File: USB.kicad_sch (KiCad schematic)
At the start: 40 parts, among them J5 USB_C_Receptacle, J6 USB_C_Receptacle, Q1 DMN32D2LFB4, Q2 DMN32D2LFB4, U10 TPD4EUSB30, U11 TPD4EUSB30, U12 TPD4EUSB30, U14 TPD4EUSB30, U15 TS3USB221, U17 TS3USB221, U19 TS3USB221, U20 TPD6S300A, U21 TPD6S300A, U7 FUSB340TMX, U9 FUSB340TMX

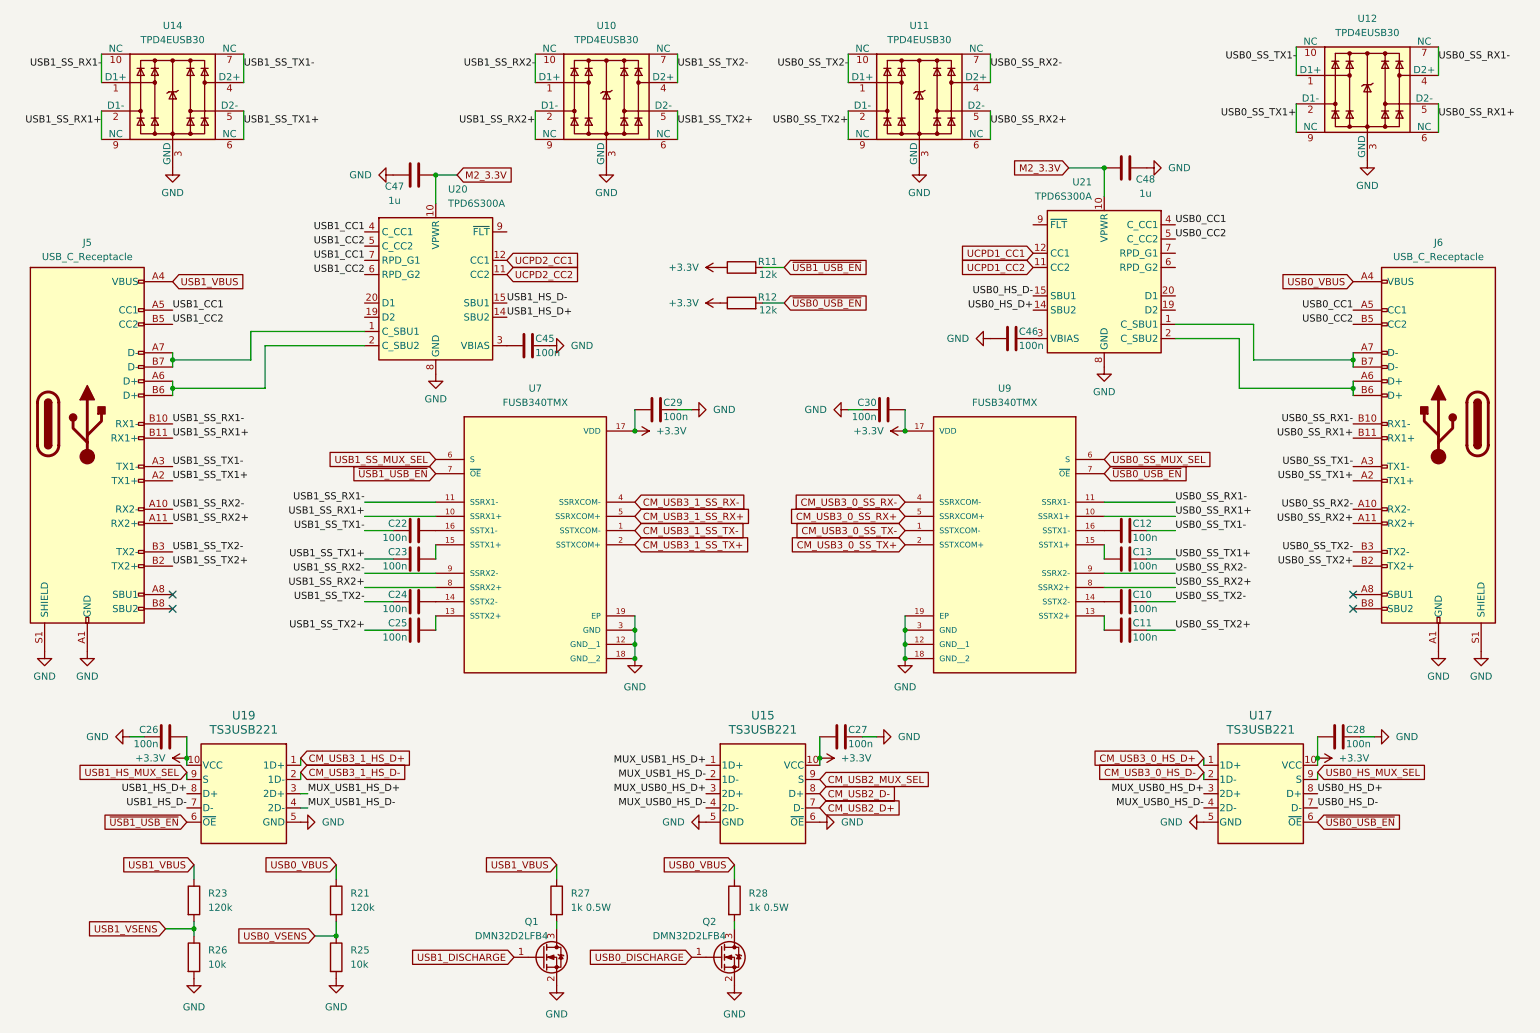
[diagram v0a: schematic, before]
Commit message: WIP
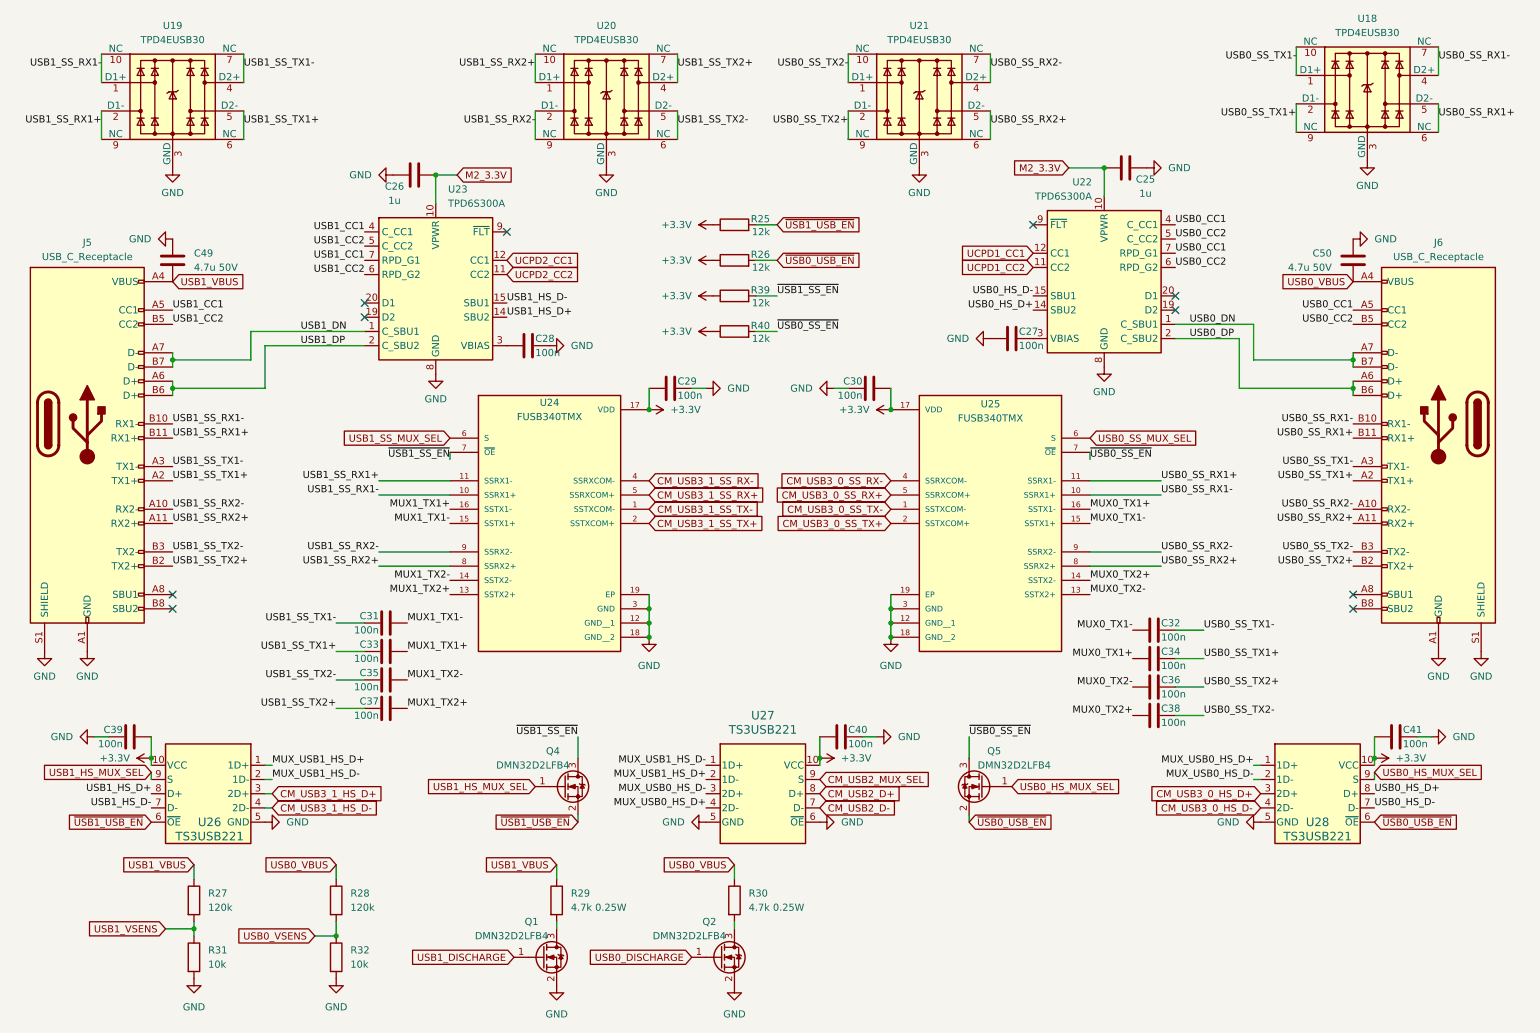
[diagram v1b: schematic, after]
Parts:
- removed C10, C11, C12, C13, C22, C23, C24, C25: 100n, Capacitor_SMD:C_0402_1005Metric, symbol Device:C
- added C31, C32, C33, C34, C35, C36, C37, C38: 100n, Capacitor_SMD:C_0402_1005Metric, symbol Device:C
- added C49, C50: 4.7u 50V, Capacitor_SMD:C_0805_2012Metric, symbol Device:C
- added Q4, Q5: DMN32D2LFB4, Package_DFN_QFN:Diodes_DFN1006-3, symbol Device:Q_NMOS_GSD
- added R39, R40: 12k, Resistor_SMD:R_0402_1005Metric, symbol Device:R
- R27: renamed from R23; LCSC (none) -> C25750; MPN (none) -> 0402WGF1203TCE; Manufacturer (none) -> Uniroyal
- R28: renamed from R21; LCSC (none) -> C25750; MPN (none) -> 0402WGF1203TCE; Manufacturer (none) -> Uniroyal
- R29: renamed from R27; value 1k 0.5W -> 4.7k 0.25W; LCSC (none) -> C17936; MPN (none) -> 1206W4F4701T5E; Manufacturer (none) -> Uniroyal
- R30: renamed from R28; value 1k 0.5W -> 4.7k 0.25W; LCSC (none) -> C17936; MPN (none) -> 1206W4F4701T5E; Manufacturer (none) -> Uniroyal
- R31: renamed from R26; LCSC (none) -> C25744; MPN (none) -> 0402WGF1002TCE; Manufacturer (none) -> Uniroyal
- R32: renamed from R25; LCSC (none) -> C25744; MPN (none) -> 0402WGF1002TCE; Manufacturer (none) -> Uniroyal
- U22: renamed from U21; LCSC (none) -> C2876380; MPN (none) -> TPD6S300ARUKR; Manufacturer (none) -> Texas Instruments
- U23: renamed from U20; LCSC (none) -> C2876380; MPN (none) -> TPD6S300ARUKR; Manufacturer (none) -> Texas Instruments
- U24: renamed from U7; LCSC (none) -> C478457; MPN (none) -> FUSB340TMX; Manufacturer (none) -> onsemi
- U25: renamed from U9; LCSC (none) -> C478457; MPN (none) -> FUSB340TMX; Manufacturer (none) -> onsemi
- U26: renamed from U19; LCSC (none) -> C128396; MPN (none) -> TS3USB221ARSER; Manufacturer (none) -> Texas Instruments
- U27: renamed from U15; LCSC (none) -> C128396; MPN (none) -> TS3USB221ARSER; Manufacturer (none) -> Texas Instruments
- U28: renamed from U17; LCSC (none) -> C128396; MPN (none) -> TS3USB221ARSER; Manufacturer (none) -> Texas Instruments
- renumbered C48 to C25, C47 to C26, C46 to C27, C45 to C28, C26 to C39, C27 to C40, C28 to C41, R11 to R25, R12 to R26, U12 to U18, U14 to U19, U10 to U20, U11 to U21
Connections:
- net +3.3V: now also R39.1, R40.1
- net CM_USB2_D+: now also U27.8 (D+); no longer U27.7 (D-)
- net CM_USB2_D-: now also U27.7 (D-); no longer U27.8 (D+)
- net CM_USB3_0_HS_D+: now also U28.3 (2D+); no longer U28.1 (1D+)
- net CM_USB3_0_HS_D-: now also U28.4 (2D-); no longer U28.2 (1D-)
- net CM_USB3_1_HS_D+: now also U26.3 (2D+); no longer U26.1 (1D+)
- net CM_USB3_1_HS_D-: now also U26.4 (2D-); no longer U26.2 (1D-)
- net GND: now also C49.1, C50.1
- net MUX_USB0_HS_D+: now also U27.4 (2D-), U28.1 (1D+); no longer U27.3 (2D+), U28.3 (2D+)
- net MUX_USB0_HS_D-: now also U27.3 (2D+), U28.2 (1D-); no longer U27.4 (2D-), U28.4 (2D-)
- net MUX_USB1_HS_D+: now also U26.1 (1D+), U27.2 (1D-); no longer U26.3 (2D+), U27.1 (1D+)
- net MUX_USB1_HS_D-: now also U26.2 (1D-), U27.1 (1D+); no longer U26.4 (2D-), U27.2 (1D-)
- net USB0_CC1: now also U22.7 (RPD_G1)
- net USB0_CC2: now also U22.6 (RPD_G2)
- net USB0_HS_MUX_SEL: now also Q5.1 (G)
- net USB0_SS_RX1+: now also U25.11 (SSRX1-); no longer U25.10 (SSRX1+)
- net USB0_SS_RX1-: now also U25.10 (SSRX1+); no longer U25.11 (SSRX1-)
- net USB0_SS_TX1+: now also C34.1
- net USB0_SS_TX1-: now also C32.1
- net USB0_SS_TX2+: now also C36.1
- net USB0_SS_TX2-: now also C38.1
- net USB0_VBUS: now also C50.2
- net USB1_HS_MUX_SEL: now also Q4.1 (G)
- net USB1_SS_RX1+: now also U24.11 (SSRX1-); no longer U24.10 (SSRX1+)
- net USB1_SS_RX1-: now also U24.10 (SSRX1+); no longer U24.11 (SSRX1-)
- net USB1_SS_RX2+: now also U20.1 (D1+), U20.10 (NC); no longer U20.2 (D1-), U20.9 (NC)
- net USB1_SS_RX2-: now also U20.2 (D1-), U20.9 (NC); no longer U20.1 (D1+), U20.10 (NC)
- net USB1_SS_TX1+: now also C33.1
- net USB1_SS_TX1-: now also C31.1
- net USB1_SS_TX2+: now also U20.4 (D2+), U20.7 (NC), C37.1; no longer U20.5 (D2-), U20.6 (NC)
- net USB1_SS_TX2-: now also U20.5 (D2-), U20.6 (NC), C35.1; no longer U20.4 (D2+), U20.7 (NC)
- net USB1_VBUS: now also C49.2
- net ~{USB0_USB_EN}: now also Q5.2 (S); no longer U25.7 (~{OE})
- net ~{USB1_USB_EN}: now also Q4.2 (S); no longer U24.7 (~{OE})
- net MUX0_TX2+: now reaches U25.14 (SSTX2-)
- net MUX0_TX2+: now also C38.2
- net MUX0_TX1+: now reaches U25.16 (SSTX1-)
- net MUX0_TX1+: now also C34.2
- net USB0_DN: now reaches J6.A7 (D-), J6.B7 (D-), U22.1 (C_SBU1)
- net USB0_DP: now reaches J6.A6 (D+), J6.B6 (D+), U22.2 (C_SBU2)
- net MUX1_TX2+: now reaches U24.13 (SSTX2+)
- net MUX1_TX2+: now also C37.2
- net MUX0_TX2-: now reaches U25.13 (SSTX2+)
- net MUX0_TX2-: now also C36.2
- net MUX0_TX1-: now reaches U25.15 (SSTX1+)
- net MUX0_TX1-: now also C32.2
- net MUX1_TX1+: now reaches U24.16 (SSTX1-)
- net MUX1_TX1+: now also C33.2
- net USB1_DN: now reaches J5.A7 (D-), J5.B7 (D-), U23.1 (C_SBU1)
- net USB1_DP: now reaches J5.A6 (D+), J5.B6 (D+), U23.2 (C_SBU2)
- net MUX1_TX1-: now reaches U24.15 (SSTX1+)
- net MUX1_TX1-: now also C31.2
- net MUX1_TX2-: now reaches U24.14 (SSTX2-)
- net MUX1_TX2-: now also C35.2
- new net ~{USB0_SS_EN}: Q5.3 (D), R40.2, U25.7 (~{OE})
- new net ~{USB1_SS_EN}: Q4.3 (D), R39.2, U24.7 (~{OE})
- no-connect marks 4 -> 10
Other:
- title: (none) -> PiCard
- moved on the sheet: C29, C30, C39, C41, R25, R26, U24, U25, U26, U28

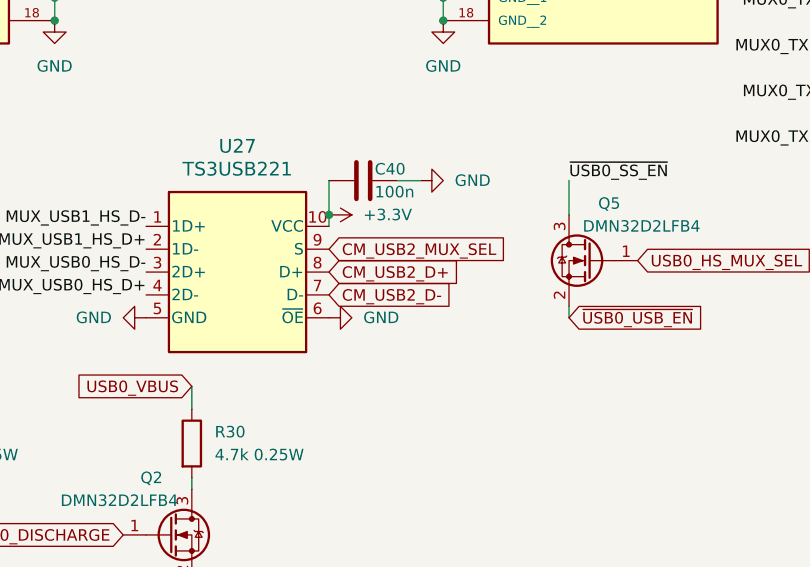
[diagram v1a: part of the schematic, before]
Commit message: final v3.0
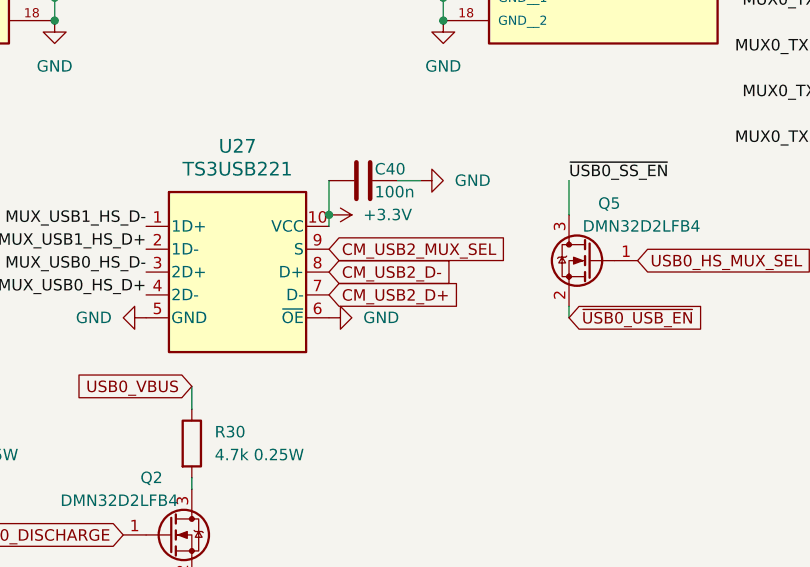
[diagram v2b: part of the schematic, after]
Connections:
- net CM_USB2_D+: now also U27.7 (D-); no longer U27.8 (D+)
- net CM_USB2_D-: now also U27.8 (D+); no longer U27.7 (D-)
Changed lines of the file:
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@@
 	(global_label "CM_USB2_D-"
 		(shape input)
-		(at 157.48 158.75 0)
+		(at 157.48 156.21 0)
 		(fields_autoplaced yes)
 		(effects
@@
 		)
 		(property "Intersheetrefs" "${INTERSHEET_REFS}"
-			(at 172.9837 158.75 0)
+			(at 172.9837 156.21 0)
 			(effects
 				(font
@@
 	(global_label "CM_USB2_D+"
 		(shape input)
-		(at 157.48 156.21 0)
+		(at 157.48 158.75 0)
 		(fields_autoplaced yes)
 		(effects
@@
 		)
 		(property "Intersheetrefs" "${INTERSHEET_REFS}"
-			(at 172.9837 156.21 0)
+			(at 172.9837 158.75 0)
 			(effects
 				(font
